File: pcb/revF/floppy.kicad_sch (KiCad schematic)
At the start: 19 parts, among them J1 FDD, U17 74LS06, U18 74LS38, U6 MB8877A

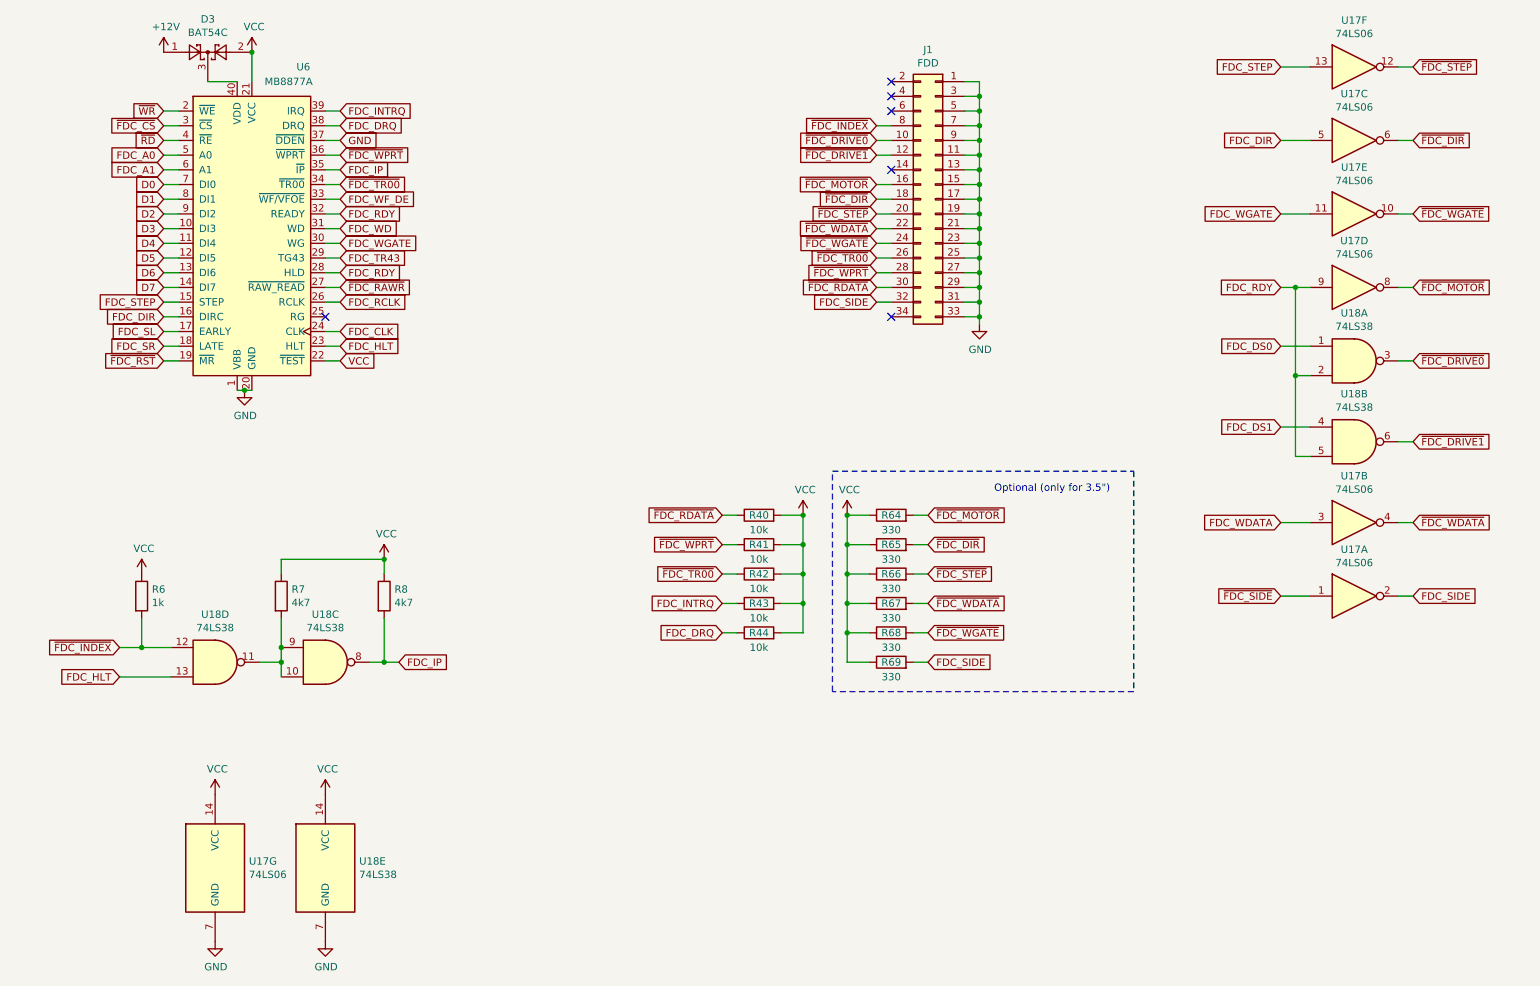
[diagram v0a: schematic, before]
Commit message: New schematics / revF
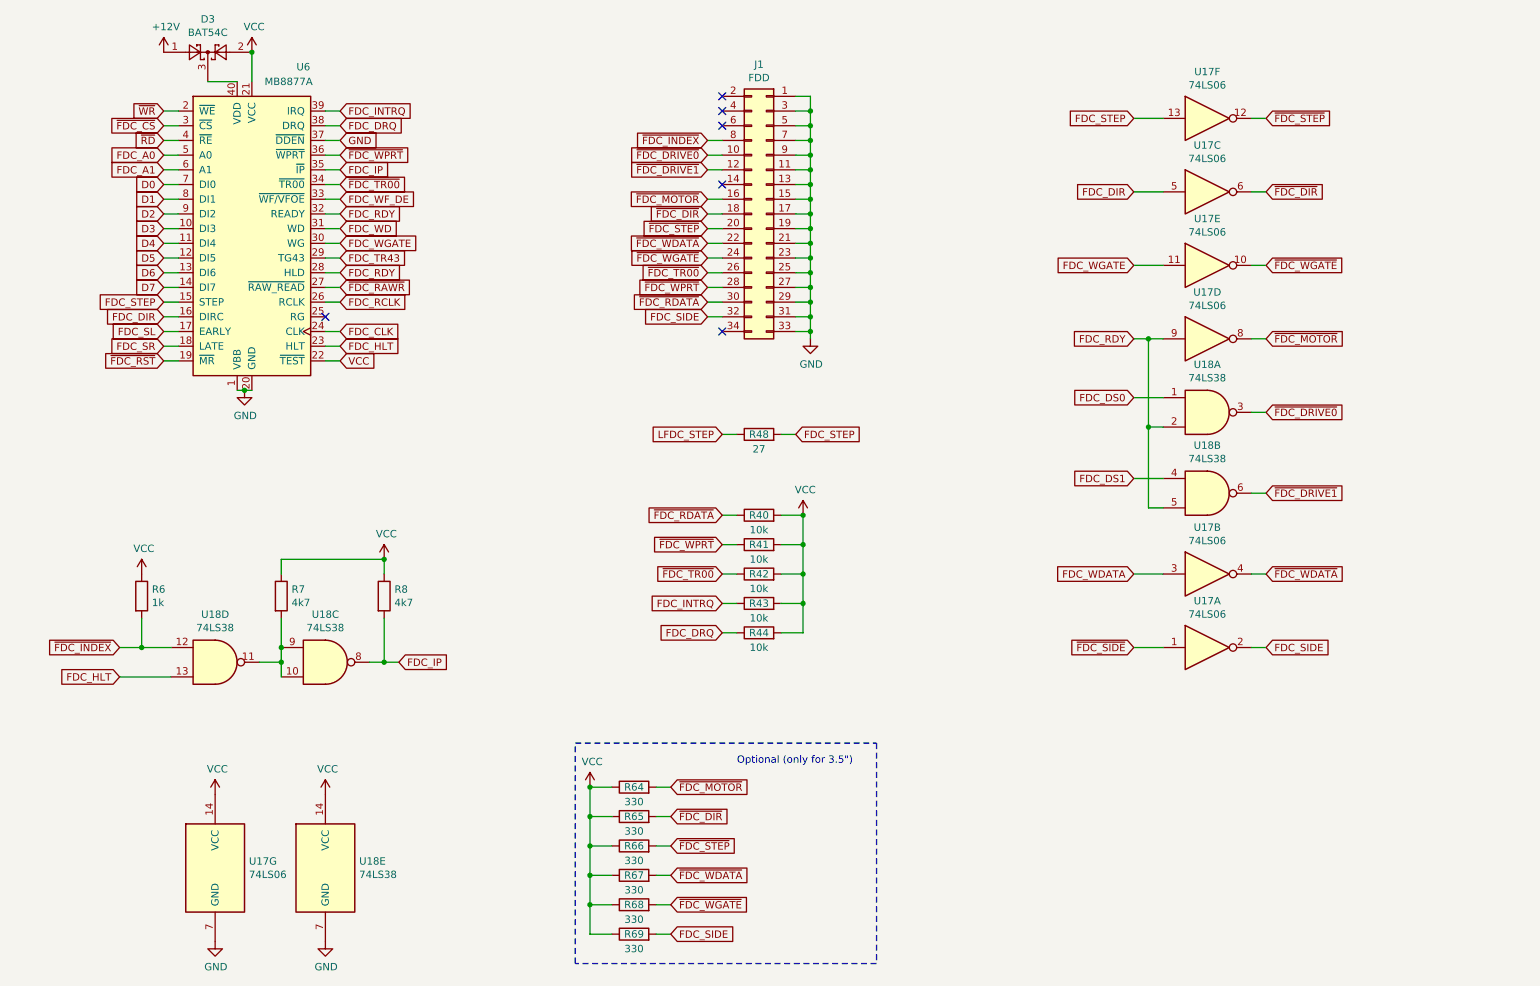
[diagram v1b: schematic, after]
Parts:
- added R48: 27, Resistor_SMD:R_0805_2012Metric_Pad1.20x1.40mm_HandSolder, symbol Device:R
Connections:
- net FDC_STEP: now also R48.2
- new net LFDC_STEP: R48.1
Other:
- moved on the sheet: J1, R64, R65, R66, R67, R68, R69, U17A, U17B, U17C, U17D, U17E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
